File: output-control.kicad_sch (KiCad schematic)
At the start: 25 parts, among them U18 ADS7828, U19 TCA9534PWR, U20 ADS7828

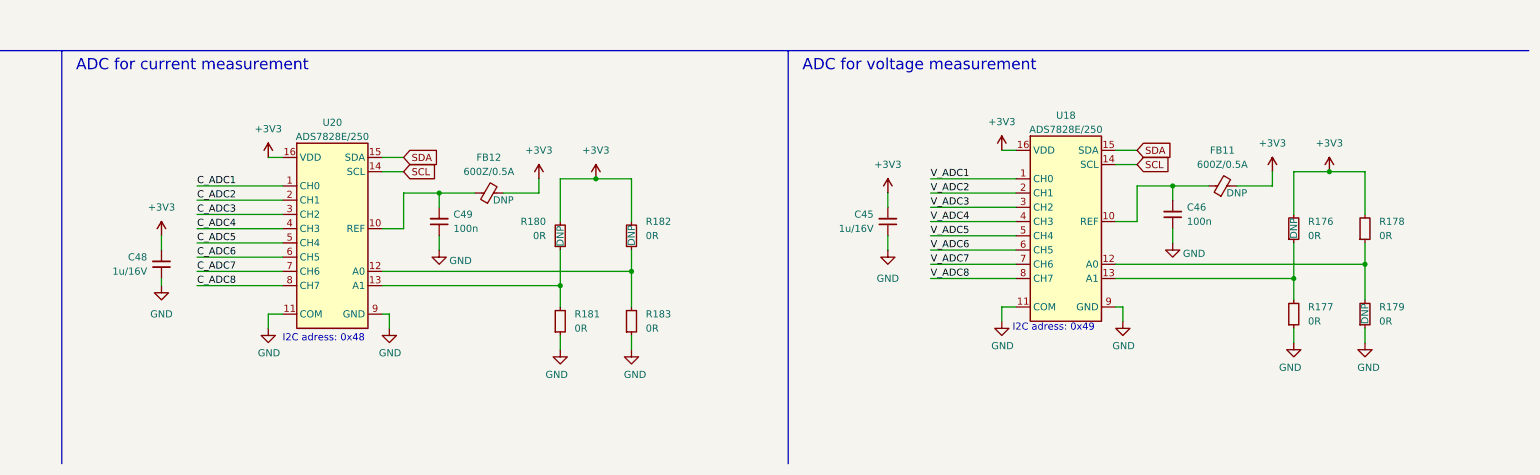
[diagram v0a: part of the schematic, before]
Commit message: 2nd part of review changes
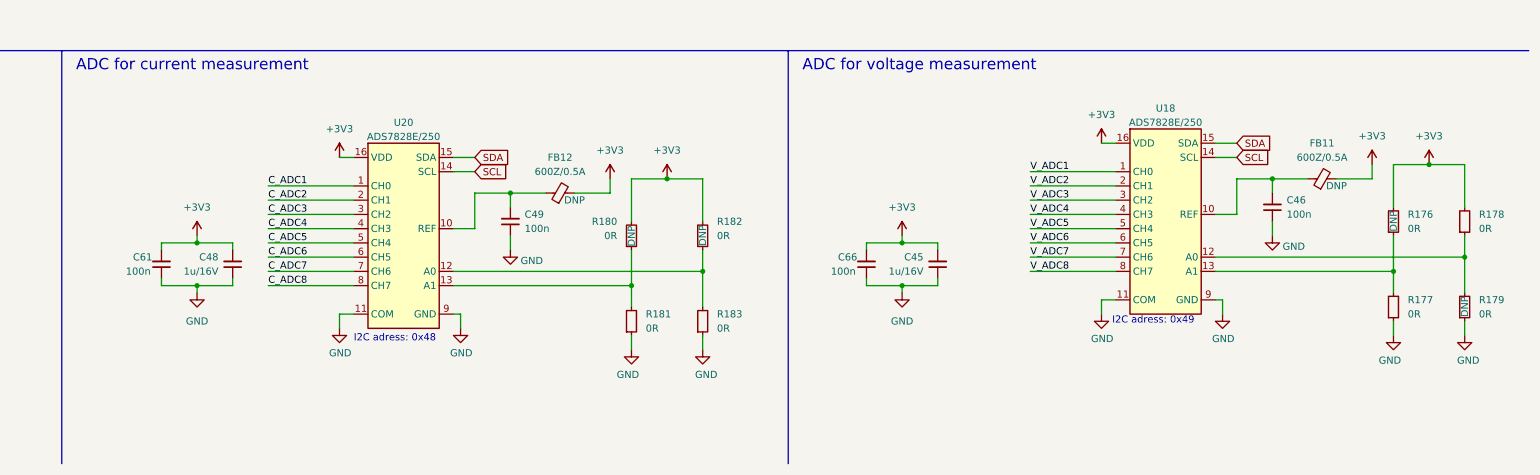
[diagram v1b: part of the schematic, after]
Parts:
- added C61, C66: C_100n_0402, antmicro-footprints:C_0402_1005Metric, symbol antmicroCapacitors0402:C_100n_0402
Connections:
- net +3V3: now also C61.2, C66.2
- net GND: now also C61.1, C66.1
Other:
- moved on the sheet: C45, C46, C48, C49, FB11, FB12, R176, R177, R178, R179, R180, R181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
